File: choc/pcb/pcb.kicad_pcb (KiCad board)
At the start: 2 copper layers, 120 x 84 mm, 67 parts, among them SW1 Switch, SW10 Switch, SW11 Switch, SW12 Switch, SW13 Switch, SW14 Switch, SW15 Switch, SW16 Switch, SW17 Switch, SW18 Switch, SW19 Switch, SW2 Switch, SW3 Switch, SW4 Switch, SW5 Switch, SW6 Switch, SW7 Switch, SW8 Switch, SW9 Switch

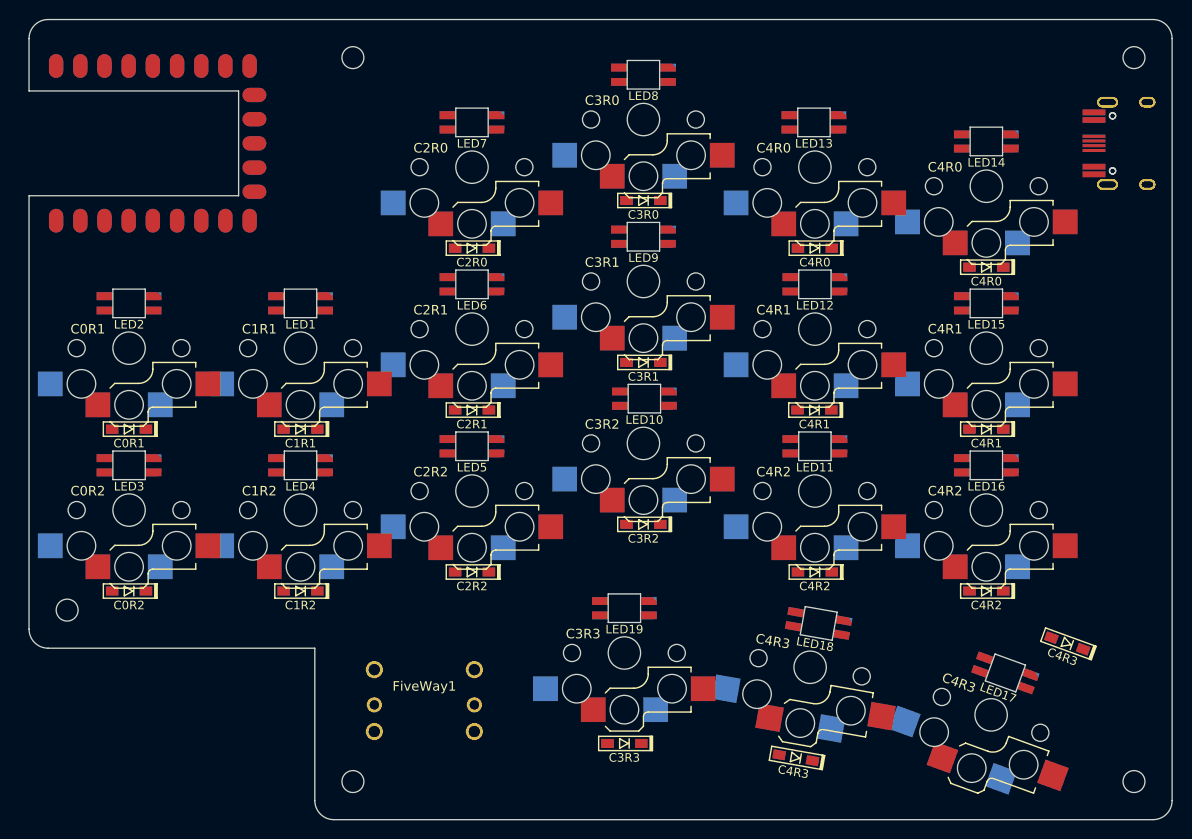
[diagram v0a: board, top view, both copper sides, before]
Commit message: small updates
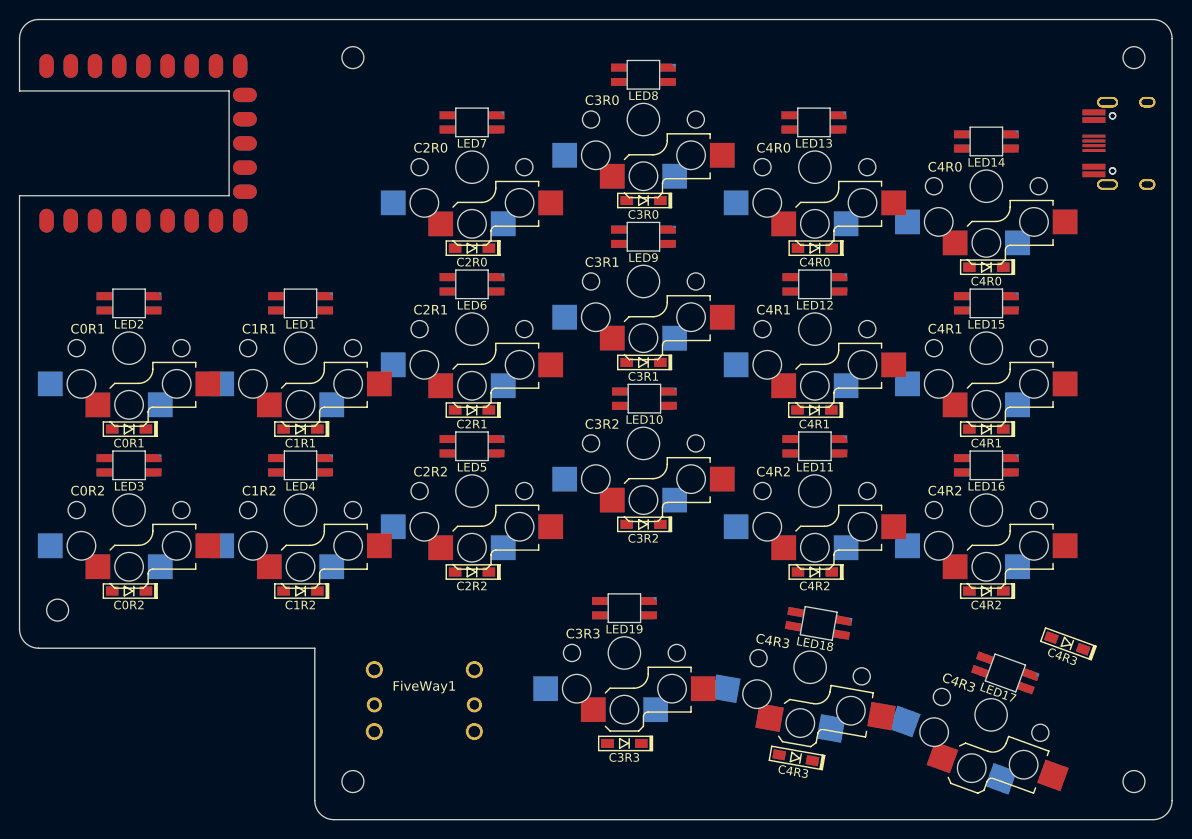
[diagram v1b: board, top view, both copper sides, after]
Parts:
- moved H3 1.00 mm to (40.0, 103.5)
- moved MCU1 1.00 mm to (49.0, 54.5)
- moved MCU2 1.00 mm to (49.0, 54.5)
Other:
- board size 120 x 84 mm -> 121 x 84 mm
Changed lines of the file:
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@@
   )
   (footprint "zzkeeb:Hole_M2" (layer "F.Cu")
-    (at 41 103.5)
+    (at 40 103.5)
     (descr "Mounting Hole 2.2mm, no annular, M2")
     (tags "mounting hole 2.2mm no annular m2")
@@
       (net 26 "col0") (pinfunction "6") (pintype "passive"))
     (model "${ZZKEEB}/models/5-WayTactileButton10mmTHT.stp"
-      (offset (xyz 5 5 0))
+      (offset (xyz 5.1 5.1 0.1))
       (scale (xyz 1 1 1))
       (rotate (xyz 0 0 -180))
     )
-    (model "${ZZKEEB}/models/5-way-concave-short.step"
+    (model "${ZZKEEB}/models/5-way-concave-short.step" hide
       (offset (xyz 0 0 6.5))
       (scale (xyz 1 1 1))
@@
   )
   (footprint "zzkeeb:MCU_rp2040-zero-smd" (layer "F.Cu")
-    (at 50 54.5 90)
+    (at 49 54.5 90)
     (property "Sheetfile" "pcb.kicad_sch")
     (property "Sheetname" "")
@@
   )
   (footprint "zzkeeb:MCU_rp2040-zero-smd" (layer "B.Cu")
-    (at 50 54.5 -90)
+    (at 49 54.5 -90)
     (property "Sheetfile" "pcb.kicad_sch")
     (property "Sheetname" "")
@@
   (gr_arc (start 69 125.5) (mid 67.585786 124.914214) (end 67 123.5)
     (stroke (width 0.1) (type default)) (layer "Edge.Cuts"))
-  (gr_line (start 37 49) (end 59 49)
+  (gr_line (start 36 49) (end 58 49)
     (stroke (width 0.1) (type default)) (layer "Edge.Cuts"))
-  (gr_line (start 37 105.5) (end 37 60)
+  (gr_line (start 36 105.5) (end 36 60)
     (stroke (width 0.1) (type default)) (layer "Edge.Cuts"))
-  (gr_line (start 59 60) (end 37 60)
+  (gr_line (start 58 60) (end 36 60)
     (stroke (width 0.1) (type default)) (layer "Edge.Cuts"))
-  (gr_line (start 39 41.5) (end 155 41.5)
+  (gr_line (start 38 41.5) (end 155 41.5)
     (stroke (width 0.1) (type default)) (layer "Edge.Cuts"))
   (gr_arc (start 157 123.5) (mid 156.414214 124.914214) (end 155 125.5)
     (stroke (width 0.1) (type default)) (layer "Edge.Cuts"))
-  (gr_line (start 59 49) (end 59 60)
+  (gr_line (start 58 49) (end 58 60)
     (stroke (width 0.1) (type default)) (layer "Edge.Cuts"))
   (gr_line (start 67 107.5) (end 67 123.5)
     (stroke (width 0.1) (type default)) (layer "Edge.Cuts"))
-  (gr_arc (start 37 43.5) (mid 37.585786 42.085786) (end 39 41.5)
+  (gr_arc (start 36 43.5) (mid 36.585786 42.085786) (end 38 41.5)
     (stroke (width 0.1) (type default)) (layer "Edge.Cuts"))
-  (gr_line (start 39 107.5) (end 67 107.5)
+  (gr_line (start 38 107.5) (end 67 107.5)
     (stroke (width 0.1) (type default)) (layer "Edge.Cuts"))
   (gr_line (start 155 125.5) (end 69 125.5)
     (stroke (width 0.1) (type default)) (layer "Edge.Cuts"))
-  (gr_line (start 37 49) (end 37 43.5)
+  (gr_line (start 36 49) (end 36 43.5)
     (stroke (width 0.1) (type default)) (layer "Edge.Cuts"))
-  (gr_arc (start 39 107.5) (mid 37.585786 106.914214) (end 37 105.5)
+  (gr_arc (start 38 107.5) (mid 36.585786 106.914214) (end 36 105.5)
     (stroke (width 0.1) (type default)) (layer "Edge.Cuts"))
 )
